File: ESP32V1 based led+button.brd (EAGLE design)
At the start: 92.4 x 95.2 mm, 11 parts

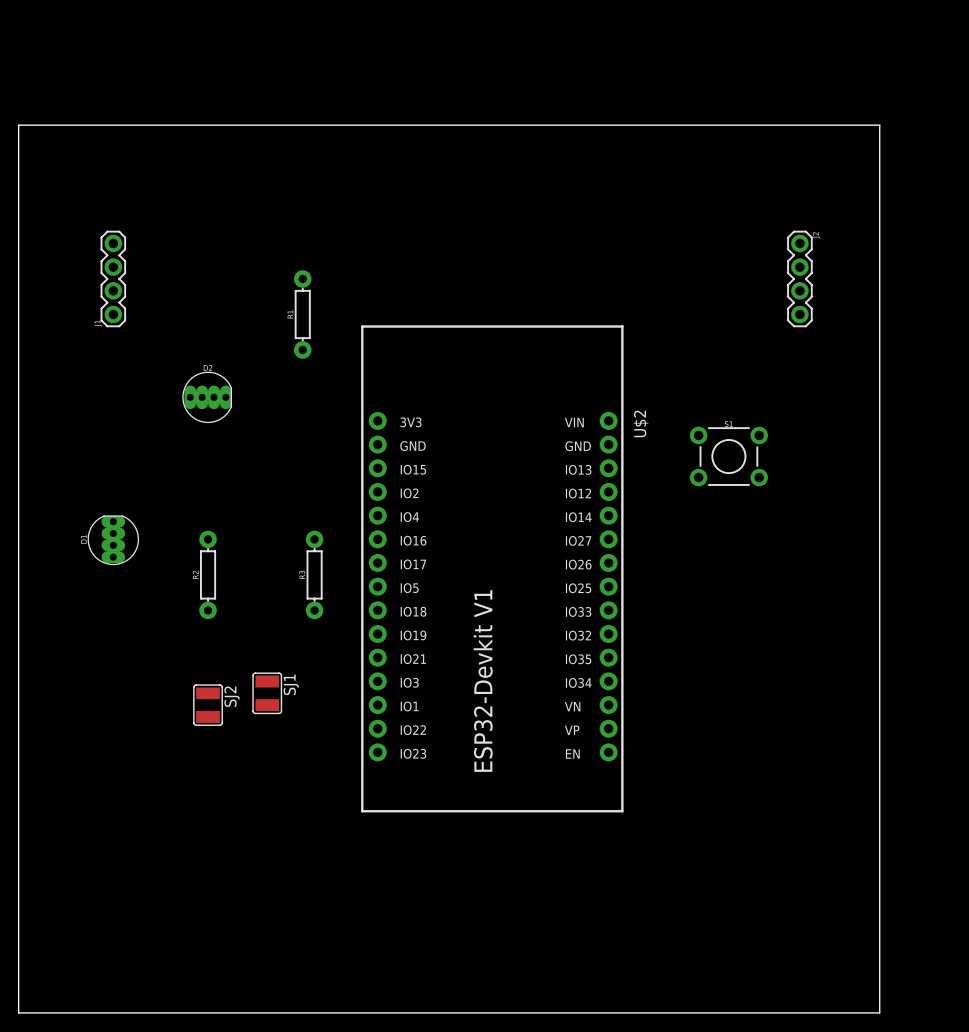
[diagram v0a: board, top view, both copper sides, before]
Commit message: edited files
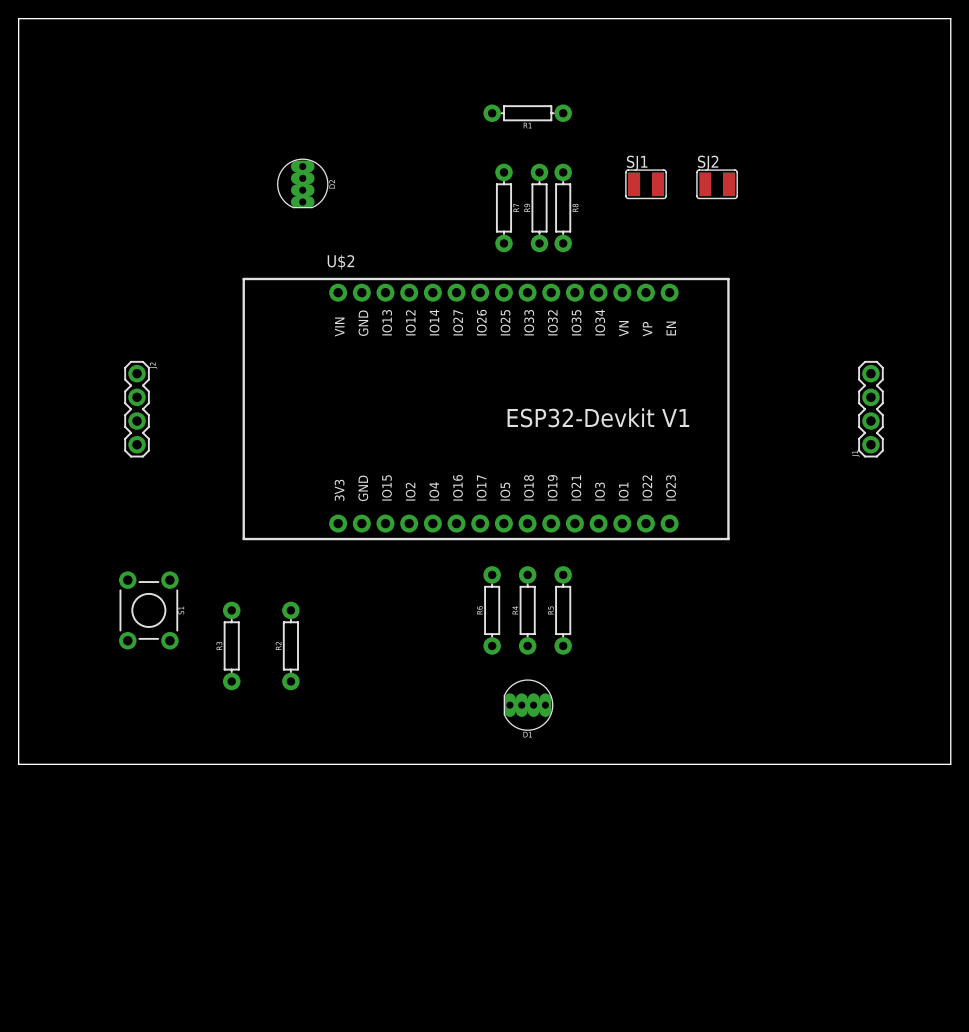
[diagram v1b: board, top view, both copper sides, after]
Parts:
- added R4, R5, R6, R7, R8, R9: 330, SparkFun-Resistors:AXIAL-0.3
- moved J1 82.5 mm to (91.4, 34.3)
- moved SJ2 78.1 mm to (74.9, 62.2), turned to 0 degrees
- moved J2 72.5 mm to (12.7, 41.9)
- moved SJ1 68.1 mm to (67.3, 62.2), turned to 0 degrees
- moved S1 64.4 mm to (14.0, 16.5), turned to 270 degrees
- moved D1 47.9 mm to (54.6, 6.35), turned to 180 degrees
- moved R1 32.4 mm to (54.6, 69.8), turned to 180 degrees
- moved U$2 25.9 mm to (57.1, 39.4), turned to 0 degrees
- moved D2 25.0 mm to (30.5, 62.2), turned to 270 degrees
- moved R2 11.7 mm to (29.2, 12.7)
- moved R3 11.7 mm to (22.9, 12.7)
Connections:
- new net B1: R5.P$2, U$2.10
- new net B2: R8.P$2, U$2.21
- new net G1: R4.P$2, U$2.9
- new net G2: R9.P$2, U$2.22
- new net N$10: D2.1, R7.P$1
- new net N$17: D2.3, R9.P$1
- new net R1: R6.P$2, U$2.8
- new net R2: R7.P$2, U$2.23
- new net RX0: J1.3, U$2.12
- new net RX2: J2.3, U$2.6
- new net TX0: J1.2, U$2.13
- new net TX2: J2.2, U$2.7
- net GND: no longer U$2.28
- net N$5: now also D1.3, R4.P$1; no longer J1.3
- net N$6: now also D1.4, R5.P$1; no longer J1.2
- net N$7: now also D1.1, R6.P$1; no longer J2.2
- net N$8: now also D2.4, R8.P$1; no longer J2.3
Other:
- board size 92.4 x 95.2 mm -> 100 x 80 mm
